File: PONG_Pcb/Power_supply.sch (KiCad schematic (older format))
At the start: 12 parts, among them J2 Input_Supply+5V, U2 LD1117S33TR_SOT223

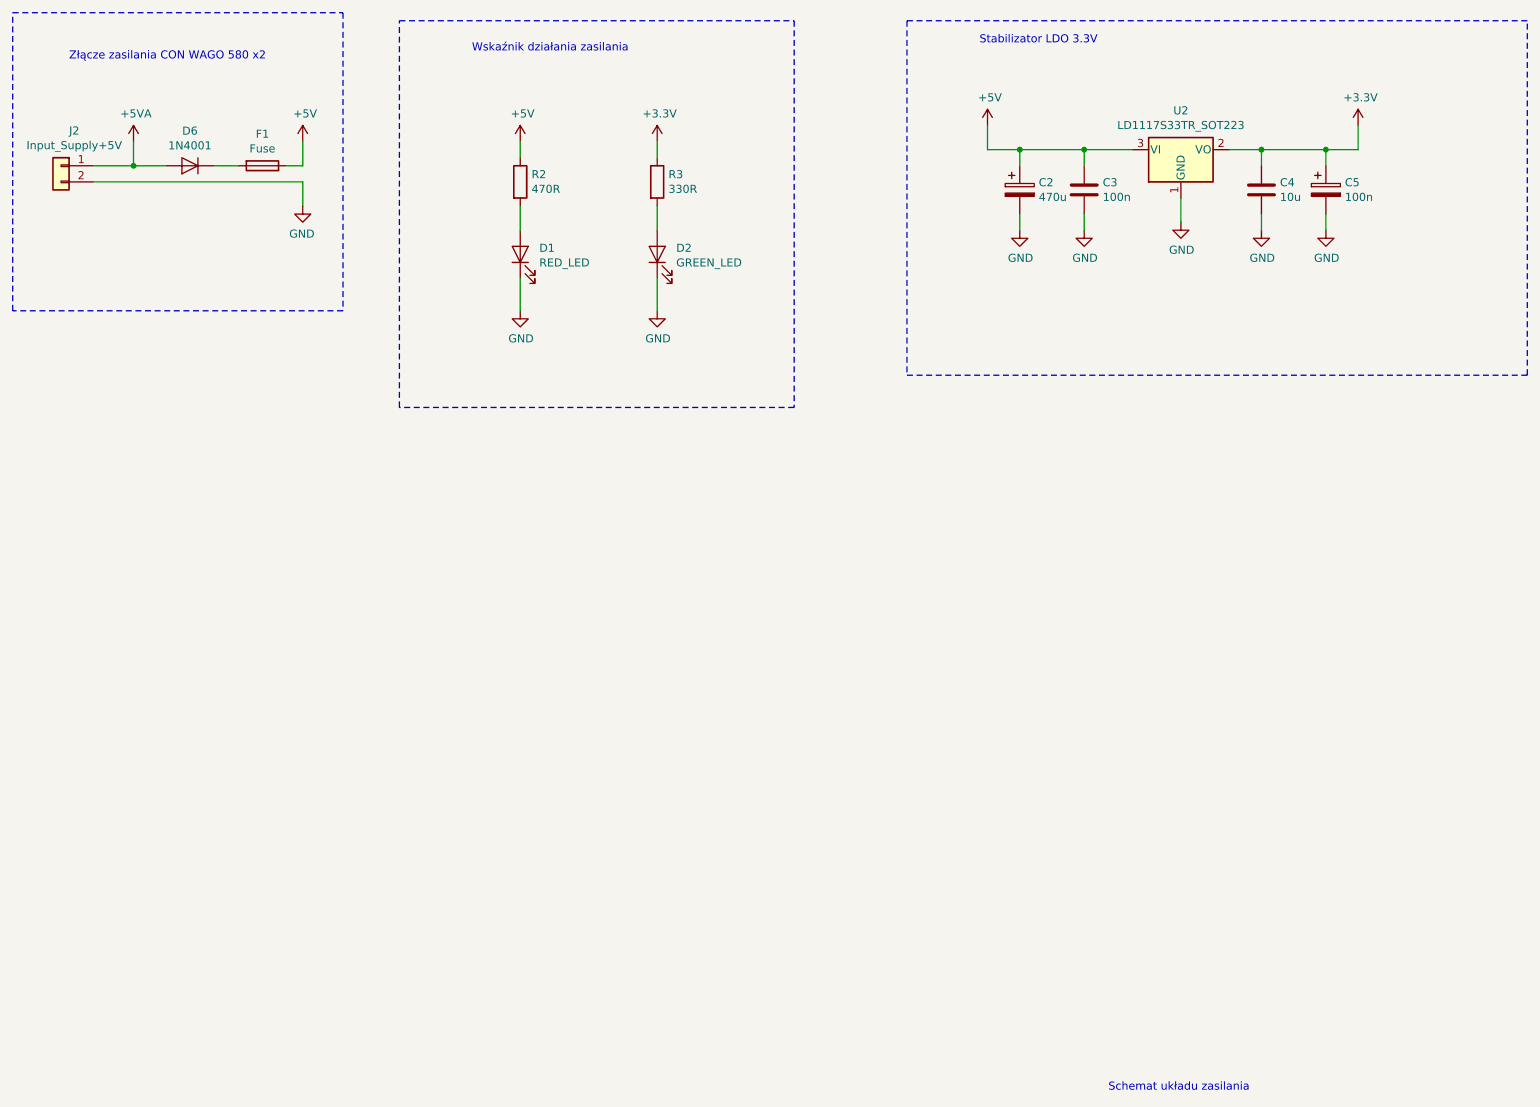
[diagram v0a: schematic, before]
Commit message: poprawki koncowe
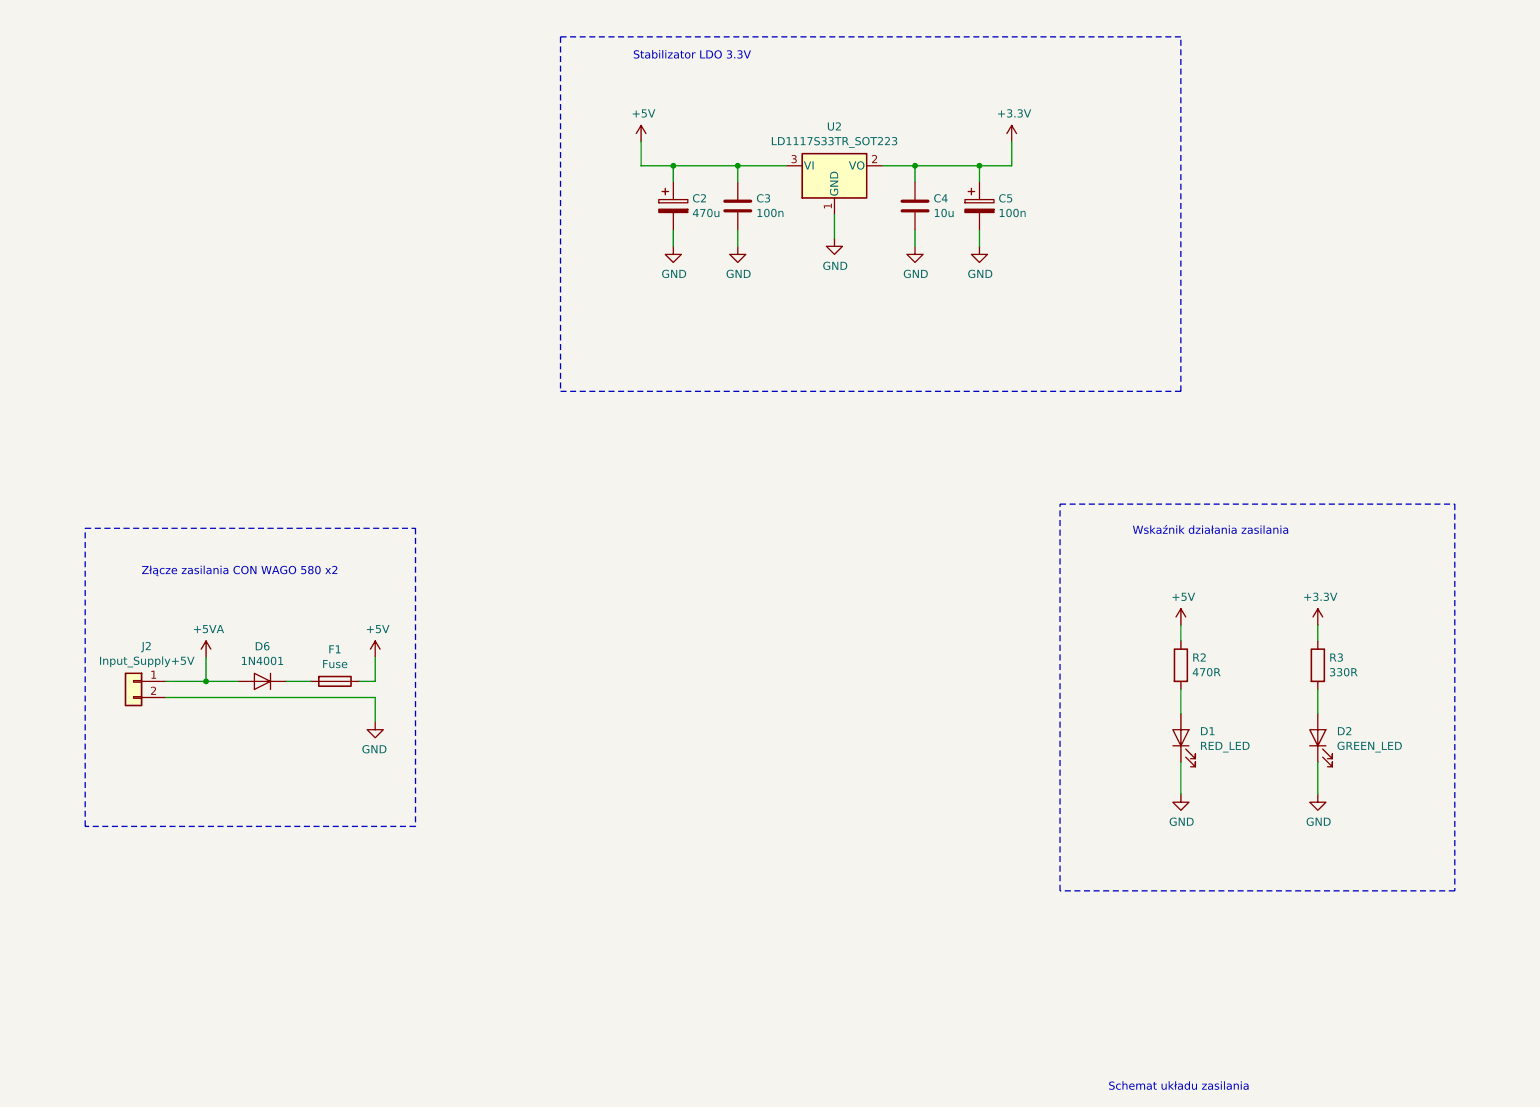
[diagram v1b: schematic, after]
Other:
- moved on the sheet: C2, C3, C4, C5, D1, D2, D6, F1, J2, R2, R3, U2
